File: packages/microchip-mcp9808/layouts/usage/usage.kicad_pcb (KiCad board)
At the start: 2 copper layers, 5 parts

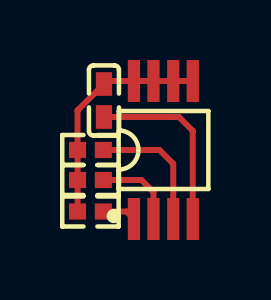
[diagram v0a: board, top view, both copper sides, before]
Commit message: fix some more packages
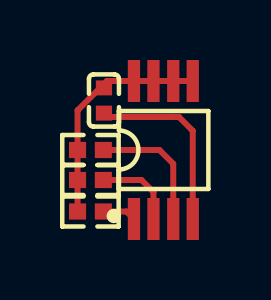
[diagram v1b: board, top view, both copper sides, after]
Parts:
- C1: value 100nF ±10% 16V X7R -> {8.99999998509884e-08..1.1000000014901162e-07}F
- R1, R2, R3: value 10kΩ ±1% 62.5mW -> {10000.0±1.0%}Ω
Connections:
- net GND renamed lv
- net VCC renamed 7

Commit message: review tool updates
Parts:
- C1: value {8.99999998509884e-08..1.1000000014901162e-07}F -> 1.0000000000000001e-07F
- R1, R2, R3: value {10000.0±1.0%}Ω -> 10000.0Ω
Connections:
- net 7 renamed hv
